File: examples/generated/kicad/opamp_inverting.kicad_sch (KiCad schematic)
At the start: 6 parts

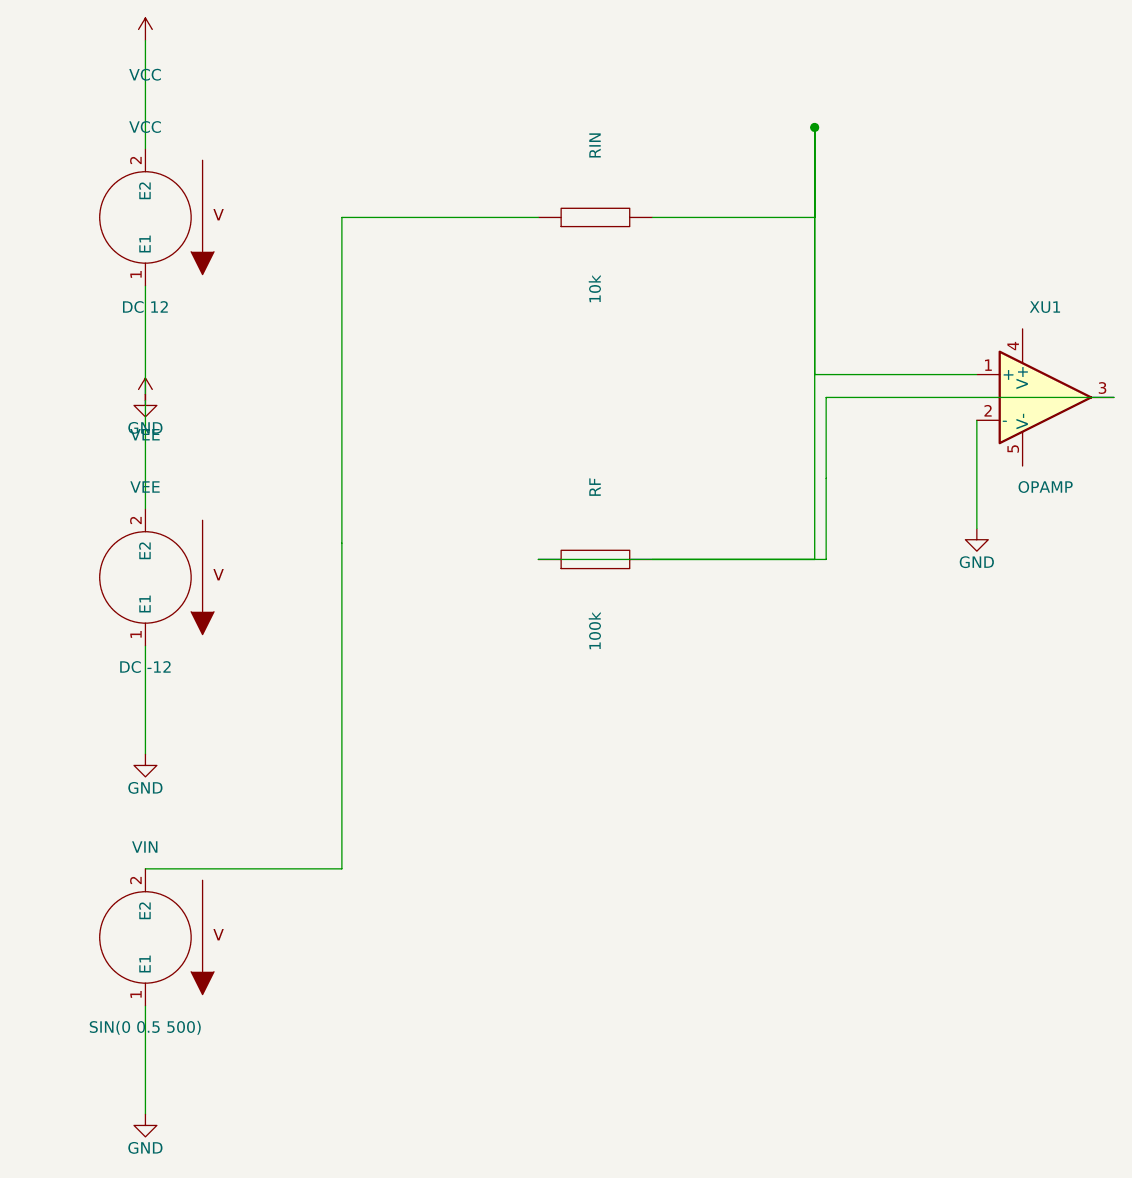
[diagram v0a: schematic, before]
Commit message: Attempt to correct strange wiring.
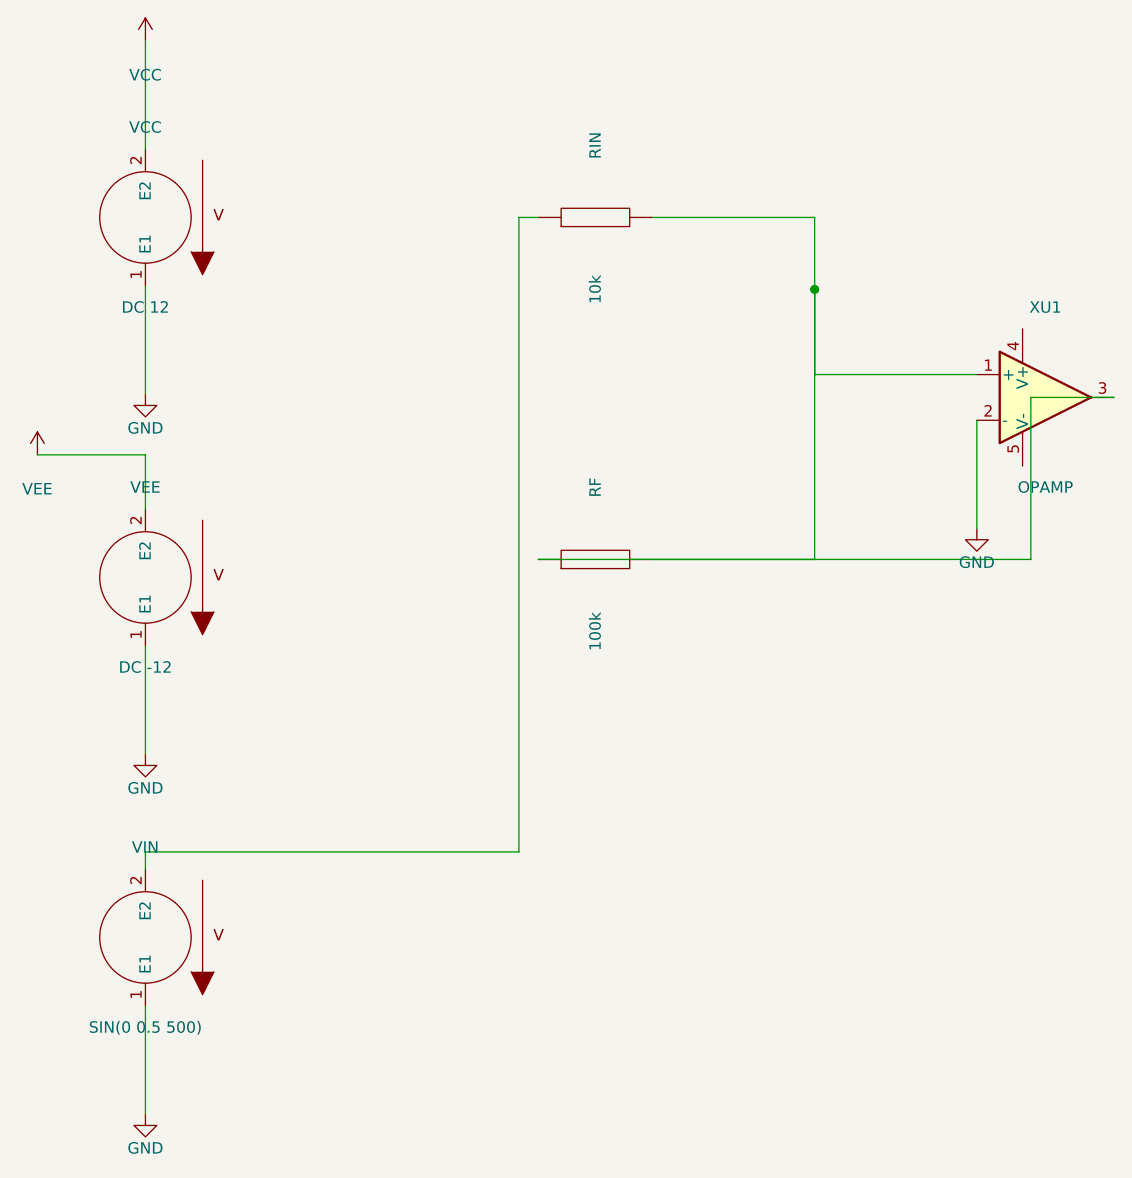
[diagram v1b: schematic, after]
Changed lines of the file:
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@@
     )
   )
-  (symbol (lib_id "VCC") (at 50.00 90.38 0) (unit 1)
+  (symbol (lib_id "VCC") (at 38.00 96.38 0) (unit 1)
     (in_bom yes) (on_board yes)
-    (property "Reference" "#PWR0003" (at 50.0 86.57 0)
+    (property "Reference" "#PWR0003" (at 38.0 92.57 0)
       (effects (font (size 1.27 1.27)) hide)
     )
-    (property "Value" "VEE" (at 50.0 94.19 0)
+    (property "Value" "VEE" (at 38.0 100.19 0)
       (effects (font (size 1.27 1.27)))
     )
@@
     (stroke (width 0) (type solid) (color 0 0 0 0))
   )
-  (wire (pts (xy 50.00 102.38) (xy 50.00 90.38))
+  (wire (pts (xy 50.00 102.38) (xy 50.00 96.38))
+    (stroke (width 0) (type solid) (color 0 0 0 0))
+  )
+  (wire (pts (xy 50.00 96.38) (xy 38.00 96.38))
     (stroke (width 0) (type solid) (color 0 0 0 0))
   )
@@
     (stroke (width 0) (type solid) (color 0 0 0 0))
   )
-  (wire (pts (xy 50.00 142.38) (xy 71.83 142.38))
+  (wire (pts (xy 50.00 142.38) (xy 50.00 140.50))
     (stroke (width 0) (type solid) (color 0 0 0 0))
   )
-  (wire (pts (xy 71.83 142.38) (xy 71.83 106.19))
+  (wire (pts (xy 50.00 140.50) (xy 91.50 140.50))
     (stroke (width 0) (type solid) (color 0 0 0 0))
   )
-  (wire (pts (xy 93.65 70.00) (xy 71.83 70.00))
+  (wire (pts (xy 91.50 140.50) (xy 91.50 70.00))
     (stroke (width 0) (type solid) (color 0 0 0 0))
   )
-  (wire (pts (xy 71.83 70.00) (xy 71.83 106.19))
+  (wire (pts (xy 91.50 70.00) (xy 93.65 70.00))
     (stroke (width 0) (type solid) (color 0 0 0 0))
   )
@@
     (stroke (width 0) (type solid) (color 0 0 0 0))
   )
-  (wire (pts (xy 124.36 70.00) (xy 124.36 60.00))
+  (wire (pts (xy 124.36 70.00) (xy 124.36 78.00))
     (stroke (width 0) (type solid) (color 0 0 0 0))
   )
@@
     (stroke (width 0) (type solid) (color 0 0 0 0))
   )
-  (wire (pts (xy 124.36 108.00) (xy 124.36 60.00))
+  (wire (pts (xy 124.36 108.00) (xy 124.36 78.00))
     (stroke (width 0) (type solid) (color 0 0 0 0))
   )
@@
     (stroke (width 0) (type solid) (color 0 0 0 0))
   )
-  (wire (pts (xy 124.36 87.46) (xy 124.36 60.00))
+  (wire (pts (xy 124.36 87.46) (xy 124.36 78.00))
     (stroke (width 0) (type solid) (color 0 0 0 0))
   )
-  (wire (pts (xy 93.65 108.00) (xy 125.64 108.00))
+  (wire (pts (xy 93.65 108.00) (xy 148.38 108.00))
     (stroke (width 0) (type solid) (color 0 0 0 0))
   )
-  (wire (pts (xy 125.64 108.00) (xy 125.64 99.00))
+  (wire (pts (xy 148.38 108.00) (xy 148.38 90.00))
     (stroke (width 0) (type solid) (color 0 0 0 0))
   )
-  (wire (pts (xy 157.62 90.00) (xy 125.64 90.00))
+  (wire (pts (xy 148.38 90.00) (xy 157.62 90.00))
     (stroke (width 0) (type solid) (color 0 0 0 0))
   )
-  (wire (pts (xy 125.64 90.00) (xy 125.64 99.00))
-    (stroke (width 0) (type solid) (color 0 0 0 0))
-  )
-  (junction (at 124.36 60.00) (diameter 1.016) (color 0 0 0 0))
+  (junction (at 124.36 78.00) (diameter 1.016) (color 0 0 0 0))
   (sheet_instances
     (path "/" (page "1"))
